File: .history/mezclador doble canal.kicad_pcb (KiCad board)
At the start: 2 copper layers, 42 parts, among them J1 Conn_Coaxial, J2 Conn_Coaxial, J3 Conn_Coaxial, J4 Conn_Coaxial, J5 Conn_Coaxial, J6 Conn_Coaxial, J7 Screw_Terminal_01x02, J8 Conn_Coaxial, SW1 SW_SPST, U1 NE5532, U2 TL071

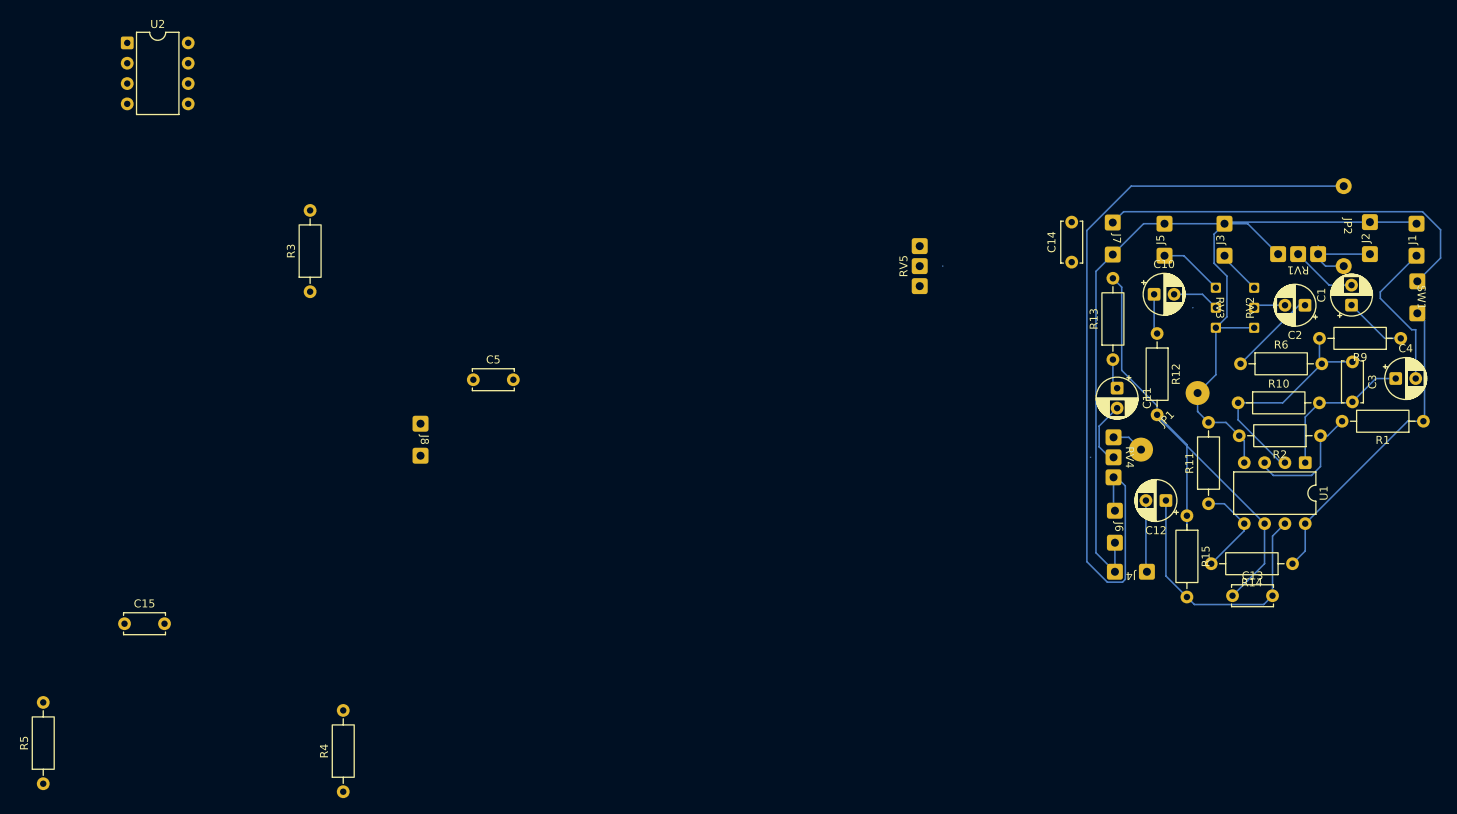
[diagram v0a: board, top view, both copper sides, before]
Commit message: acomodando componentes
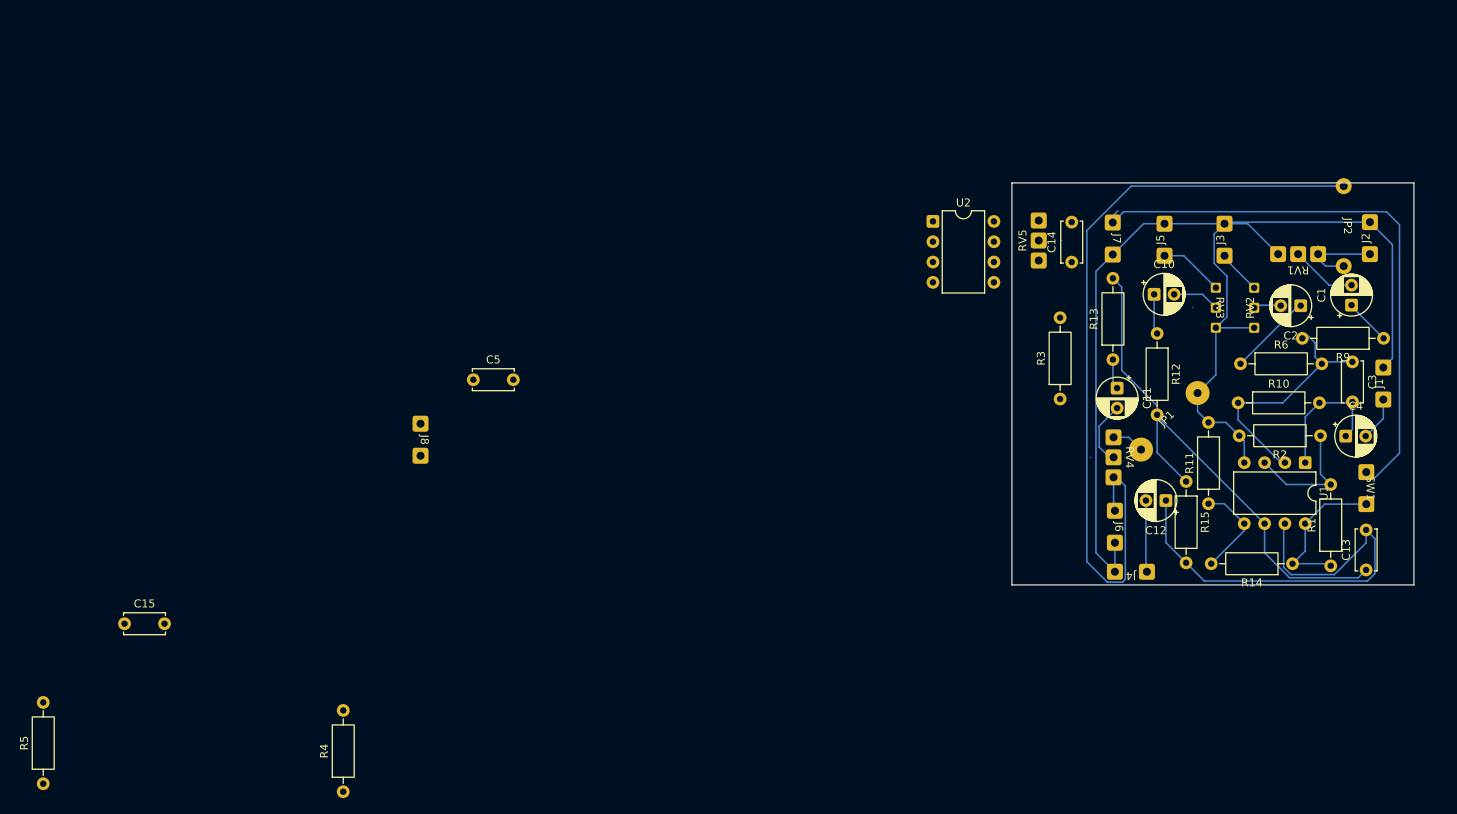
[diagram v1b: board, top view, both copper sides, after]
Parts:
- moved U2 103.2 mm to (154.1, 47.7)
- moved R3 94.7 mm to (169.9, 69.9)
- moved SW1 24.7 mm to (208.2, 81.0)
- moved R1 21.5 mm to (203.8, 90.8), turned to 90 degrees
- moved J1 18.4 mm to (210.3, 68.0)
- moved C13 17.0 mm to (208.2, 91.3), turned to 90 degrees
- moved RV5 15.2 mm to (167.3, 50.1)
- moved C4 9.53 mm to (205.7, 74.5)
- moved R15 4.28 mm to (185.7, 80.2)
- moved R9 2.15 mm to (210.4, 62.3)
- moved C2 0.54 mm to (200.0, 58.2)
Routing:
- net Net-(C12-Pad1): track 34.3 -> 59.1 mm
- net Net-(J7-Pin_1): track 50.1 -> 71.7 mm
- net VCC: track 39.7 -> 19.2 mm
- net GND: track 135.4 -> 149.3 mm
- net Net-(J1-In): track 19.4 -> 5.49 mm
- net Net-(C1-Pad1): track 7.88 -> 5.81 mm
- net Net-(C3-Pad2): track 19.5 -> 17.5 mm
- net Net-(U1B--): track 64.9 -> 66.4 mm
- net Net-(U1A--): track 30.6 -> 31.5 mm
- net Net-(U1A-+): track 15.2 -> 16.0 mm
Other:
- board outline added: 50.2 x 50.3 mm
